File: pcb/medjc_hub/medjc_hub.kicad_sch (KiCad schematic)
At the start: 40 parts, among them J1 Barrel_Jack, J2 Conn_01x02_Pin, U1 NJU7223F33, U2 NJM2747D, U3 ESP32-C3_SUPERMINI, U4 MCP3208-CI_P, U5 MERB-09, U6 MERB-09, U7 MERB-09

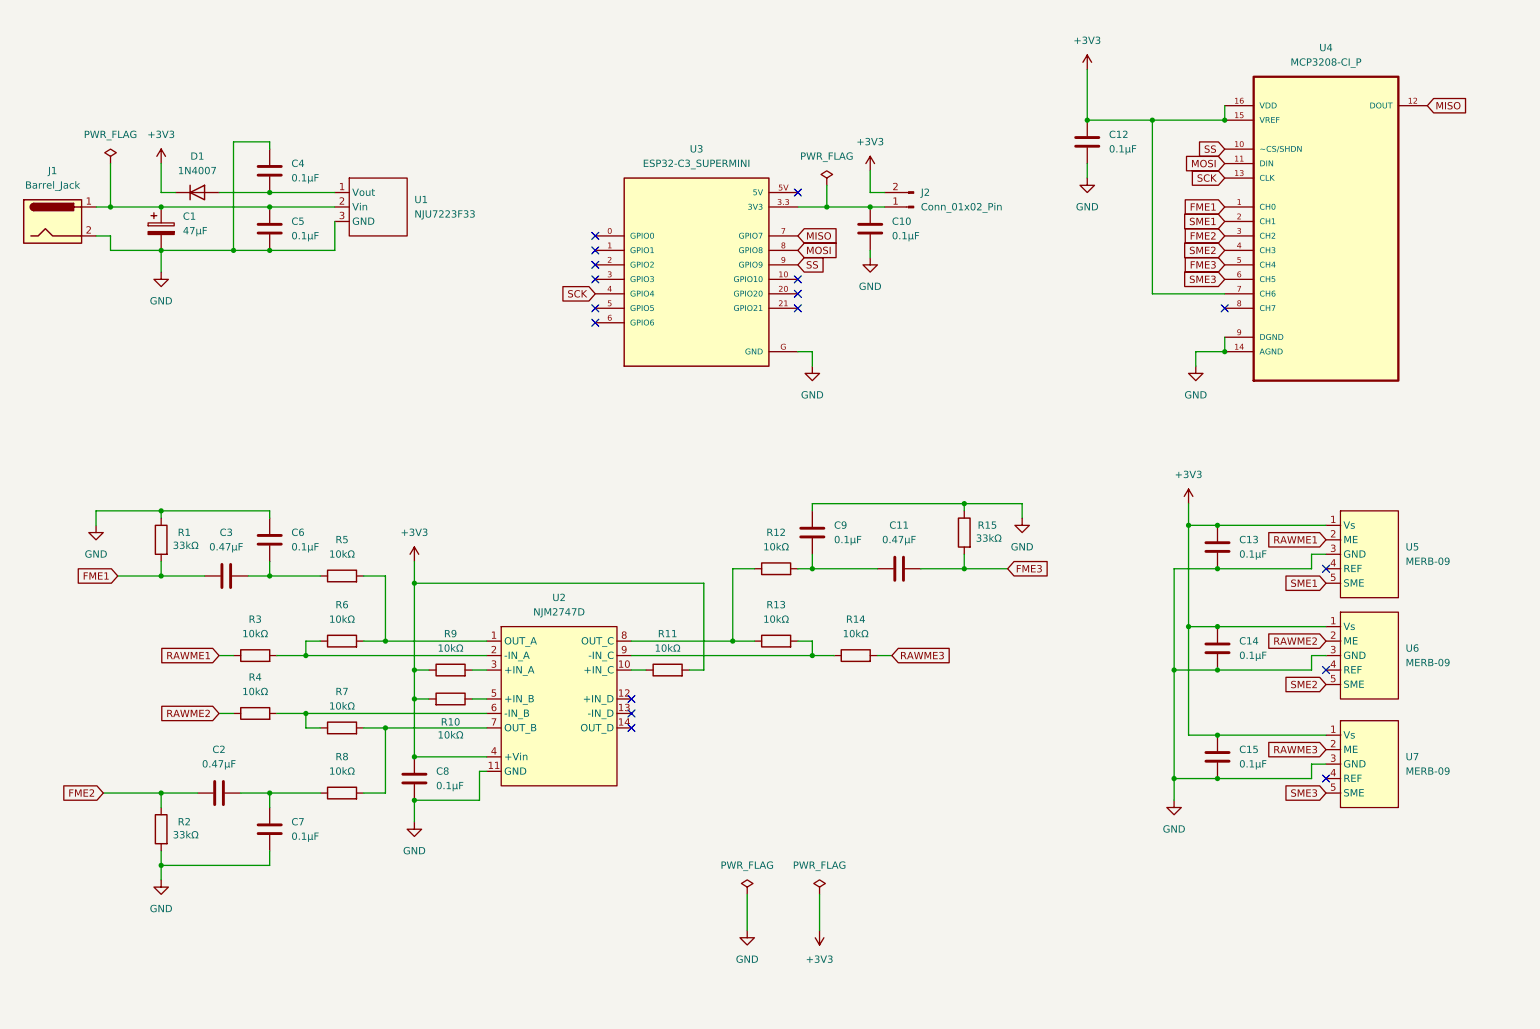
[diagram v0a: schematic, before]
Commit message: 📝 Update: 回路図を更新
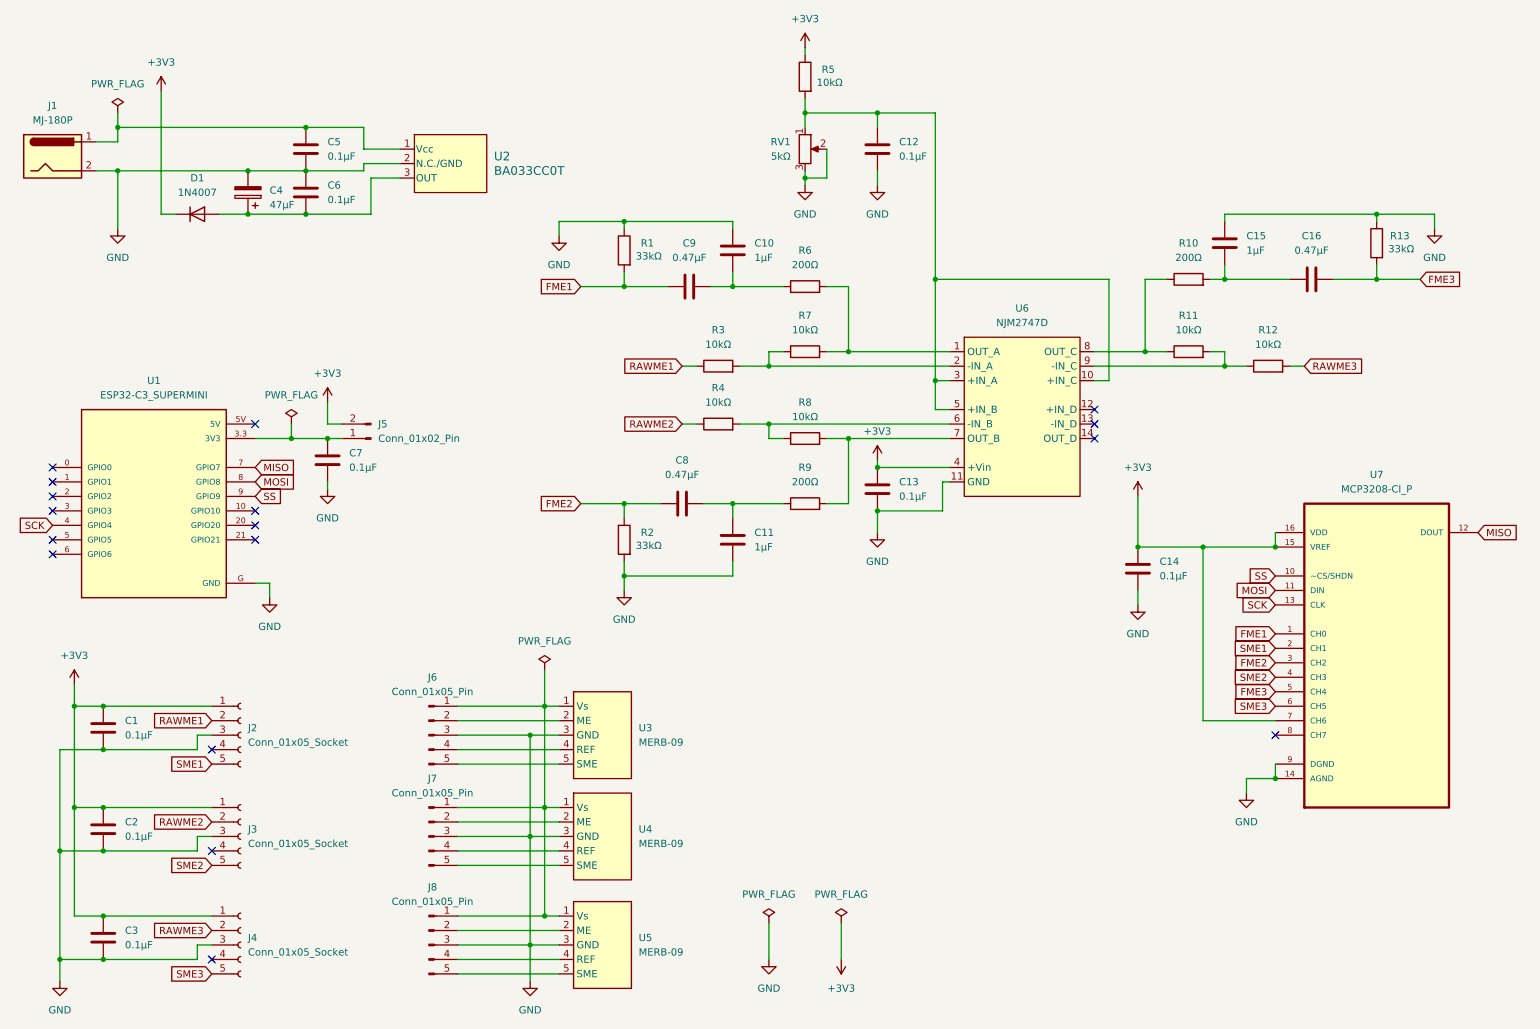
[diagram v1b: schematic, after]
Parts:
- removed C1: 47μF, symbol Device:C_Polarized
- removed C4: 0.1μF, symbol Device:C
- removed R10, R11, R9: 10kΩ, symbol Device:R
- removed U1: NJU7223F33, symbol NJU7223F33:NJU7223F33
- added C12, C6: 0.1μF, Capacitor_THT:C_Disc_D3.0mm_W2.0mm_P2.50mm, symbol Device:C
- added C4: 47μF, Capacitor_THT:CP_Radial_D5.0mm_P2.50mm, symbol Device:C_Polarized
- added J2, J3, J4: Conn_01x05_Socket, Connector_PinSocket_2.54mm:PinSocket_1x05_P2.54mm_Vertical, symbol Connector:Conn_01x05_Socket
- added J6, J7, J8: Conn_01x05_Pin, symbol Connector:Conn_01x05_Pin
- added R5: 10kΩ, Resistor_THT:R_Axial_DIN0207_L6.3mm_D2.5mm_P10.16mm_Horizontal, symbol Device:R
- added RV1: 5kΩ, GF063:GF063P, symbol Device:R_Potentiometer
- added U2: BA033CC0T, BA033CC0T:BA033CC0T, symbol BA033CC0T:BA033CC0T
- C1: renamed from C13; footprint (none) -> Capacitor_THT:C_Disc_D3.0mm_W2.0mm_P2.50mm
- C10: renamed from C6; value 0.1μF -> 1μF; footprint (none) -> Capacitor_THT:C_Disc_D3.0mm_W2.0mm_P2.50mm
- C11: renamed from C7; value 0.1μF -> 1μF; footprint (none) -> Capacitor_THT:C_Disc_D3.0mm_W2.0mm_P2.50mm
- C13: renamed from C8; footprint (none) -> Capacitor_THT:C_Disc_D3.0mm_W2.0mm_P2.50mm
- C14: renamed from C12; footprint (none) -> Capacitor_THT:C_Disc_D3.0mm_W2.0mm_P2.50mm
- C15: renamed from C9; value 0.1μF -> 1μF; footprint (none) -> Capacitor_THT:C_Disc_D3.0mm_W2.0mm_P2.50mm
- C16: renamed from C11; footprint (none) -> Capacitor_THT:C_Disc_D3.0mm_W2.0mm_P2.50mm
- C2: renamed from C14; footprint (none) -> Capacitor_THT:C_Disc_D3.0mm_W2.0mm_P2.50mm
- C3: renamed from C15; footprint (none) -> Capacitor_THT:C_Disc_D3.0mm_W2.0mm_P2.50mm
- C5: footprint (none) -> Capacitor_THT:C_Disc_D3.0mm_W2.0mm_P2.50mm
- C7: renamed from C10; footprint (none) -> Capacitor_THT:C_Disc_D3.0mm_W2.0mm_P2.50mm
- C8: renamed from C2; footprint (none) -> Capacitor_THT:C_Disc_D3.0mm_W2.0mm_P2.50mm
- C9: renamed from C3; footprint (none) -> Capacitor_THT:C_Disc_D3.0mm_W2.0mm_P2.50mm
- D1: footprint (none) -> Diode_THT:D_A-405_P10.16mm_Horizontal
- J1: value Barrel_Jack -> MJ-180P; footprint (none) -> Connector_BarrelJack:BarrelJack_Horizontal
- R1, R2, R4: footprint (none) -> Resistor_THT:R_Axial_DIN0207_L6.3mm_D2.5mm_P10.16mm_Horizontal
- R10: renamed from R12; value 10kΩ -> 200Ω; footprint (none) -> Resistor_THT:R_Axial_DIN0207_L6.3mm_D2.5mm_P10.16mm_Horizontal
- R11: renamed from R13; footprint (none) -> Resistor_THT:R_Axial_DIN0207_L6.3mm_D2.5mm_P10.16mm_Horizontal
- R12: renamed from R14; footprint (none) -> Resistor_THT:R_Axial_DIN0207_L6.3mm_D2.5mm_P10.16mm_Horizontal
- R13: renamed from R15; footprint (none) -> Resistor_THT:R_Axial_DIN0207_L6.3mm_D2.5mm_P10.16mm_Horizontal
- R3: footprint Resistor_THT:R_Box_L13.0mm_W4.0mm_P9.00mm -> Resistor_THT:R_Axial_DIN0207_L6.3mm_D2.5mm_P10.16mm_Horizontal
- R6: renamed from R5; value 10kΩ -> 200Ω; footprint (none) -> Resistor_THT:R_Axial_DIN0207_L6.3mm_D2.5mm_P10.16mm_Horizontal
- R7: renamed from R6; footprint (none) -> Resistor_THT:R_Axial_DIN0207_L6.3mm_D2.5mm_P10.16mm_Horizontal
- R8: renamed from R7; footprint (none) -> Resistor_THT:R_Axial_DIN0207_L6.3mm_D2.5mm_P10.16mm_Horizontal
- R9: renamed from R8; value 10kΩ -> 200Ω; footprint (none) -> Resistor_THT:R_Axial_DIN0207_L6.3mm_D2.5mm_P10.16mm_Horizontal
- U6: renamed from U2; footprint (none) -> Package_DIP:DIP-14_W7.62mm_Socket
- U7: renamed from U4; footprint MCP3208-CI_P:DIP254P762X432-16 -> Package_DIP:DIP-16_W7.62mm_Socket
- renumbered J2 to J5, U3 to U1, U5 to U3, U6 to U4, U7 to U5
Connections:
- net +3V3: now also J2.1 (Pin_1), J3.1 (Pin_1), J4.1 (Pin_1), R5.1; no longer U3.1 (Vs), U4.1 (Vs), U5.1 (Vs)
- net GND: now also C12.2, C4.2, C6.1, J2.3 (Pin_3), J3.3 (Pin_3), J4.3 (Pin_3), J6.3 (Pin_3), J7.3 (Pin_3), J8.3 (Pin_3), RV1.2, RV1.3, U2.2 (N.C./GND)
- net RAWME1: now also J2.2 (Pin_2); no longer U3.2 (ME)
- net RAWME2: now also J3.2 (Pin_2); no longer U4.2 (ME)
- net RAWME3: now also J4.2 (Pin_2); no longer U5.2 (ME)
- net SME1: now also J2.5 (Pin_5); no longer U3.5 (SME)
- net SME2: now also J3.5 (Pin_5); no longer U4.5 (SME)
- net SME3: now also J4.5 (Pin_5); no longer U5.5 (SME)
- net at U6.10 (+IN_C): now also U6.3 (+IN_A), U6.5 (+IN_B), C12.1, R5.2, RV1.1
- net at U4.4 (REF): now also J7.4 (Pin_4)
- net at U5.4 (REF): now also J8.4 (Pin_4)
- net at C5.1, J1.1: now also U2.1 (Vcc)
- net at D1.2 (A): now also C4.1, C6.2, U2.3 (OUT)
- net at U3.4 (REF): now also J6.4 (Pin_4)
- new net: J6.1 (Pin_1), J7.1 (Pin_1), J8.1 (Pin_1), U3.1 (Vs), U4.1 (Vs), U5.1 (Vs)
- new net: J7.2 (Pin_2), U4.2 (ME)
- new net: J7.5 (Pin_5), U4.5 (SME)
- new net: J8.2 (Pin_2), U5.2 (ME)
- new net: J8.5 (Pin_5), U5.5 (SME)
- new net: J6.2 (Pin_2), U3.2 (ME)
- new net: J6.5 (Pin_5), U3.5 (SME)
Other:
- moved on the sheet: C1, C10, C11, C13, C14, C15, C16, C2, C3, C7, C8, C9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
